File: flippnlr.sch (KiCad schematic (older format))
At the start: 90 parts, among them J1 Data In, J2 Data Out, J8 12V, U1 SN74HCS594, U10 TPL7407LA, U11 TPL7407LA, U12 SN74HCS365, U13 LD1117 3.3V, U2 SN74HCS594, U3 SN74HCS594, U4 SN74HCS594, U5 SN74HCS594, U6 TPL7407LA, U7 TPL7407LA, U8 TPL7407LA, U9 TPL7407LA

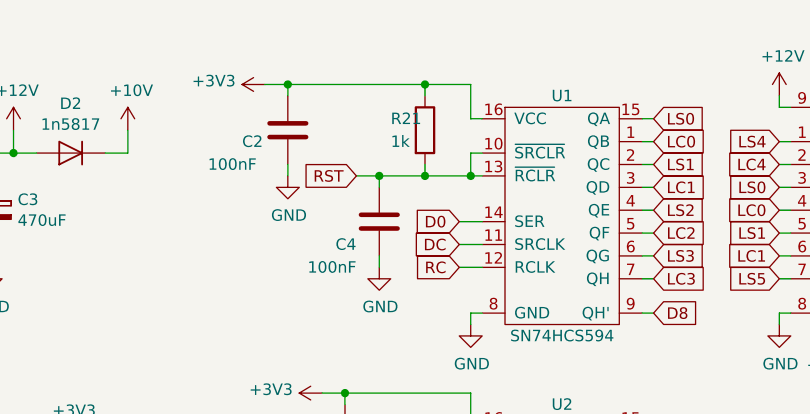
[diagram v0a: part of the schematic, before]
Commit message: first prototype
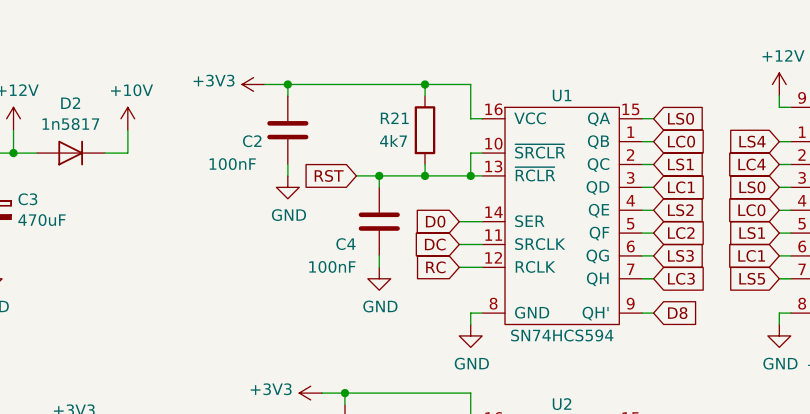
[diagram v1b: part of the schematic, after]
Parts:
- R21: value 1k -> 4k7
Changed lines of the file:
@@
 U 1 1 6131F7AE
 P 3400 1050
-F 0 "R21" H 3250 1100 50  0000 L CNN
-F 1 "1k" H 3250 1000 50  0000 L CNN
+F 0 "R21" H 3200 1100 50  0000 L CNN
+F 1 "4k7" H 3200 1000 50  0000 L CNN
 F 2 "Resistor_SMD:R_0805_2012Metric_Pad1.15x1.40mm_HandSolder" V 3330 1050 50  0001 C CNN
 F 3 "~" H 3400 1050 50  0001 C CNN
